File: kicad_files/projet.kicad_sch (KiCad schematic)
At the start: 32 parts, among them J1 STLink V3, J4 USB_B_Micro, J5 Conn_01x04, J6 Conn_01x02, Q1 BC817, Q2 BC807, Q3 NMOS, Q4 PMOS, SW1 SW_Omron_B3FS, SW2 Reset, U1 STM32G031K8Tx, U2 MCP4901, U3 LM1117MP-3.3, U4 TLV2372, U5 CD4066BM, U6 MCP4131-xxxx-P, U7 MCP4901

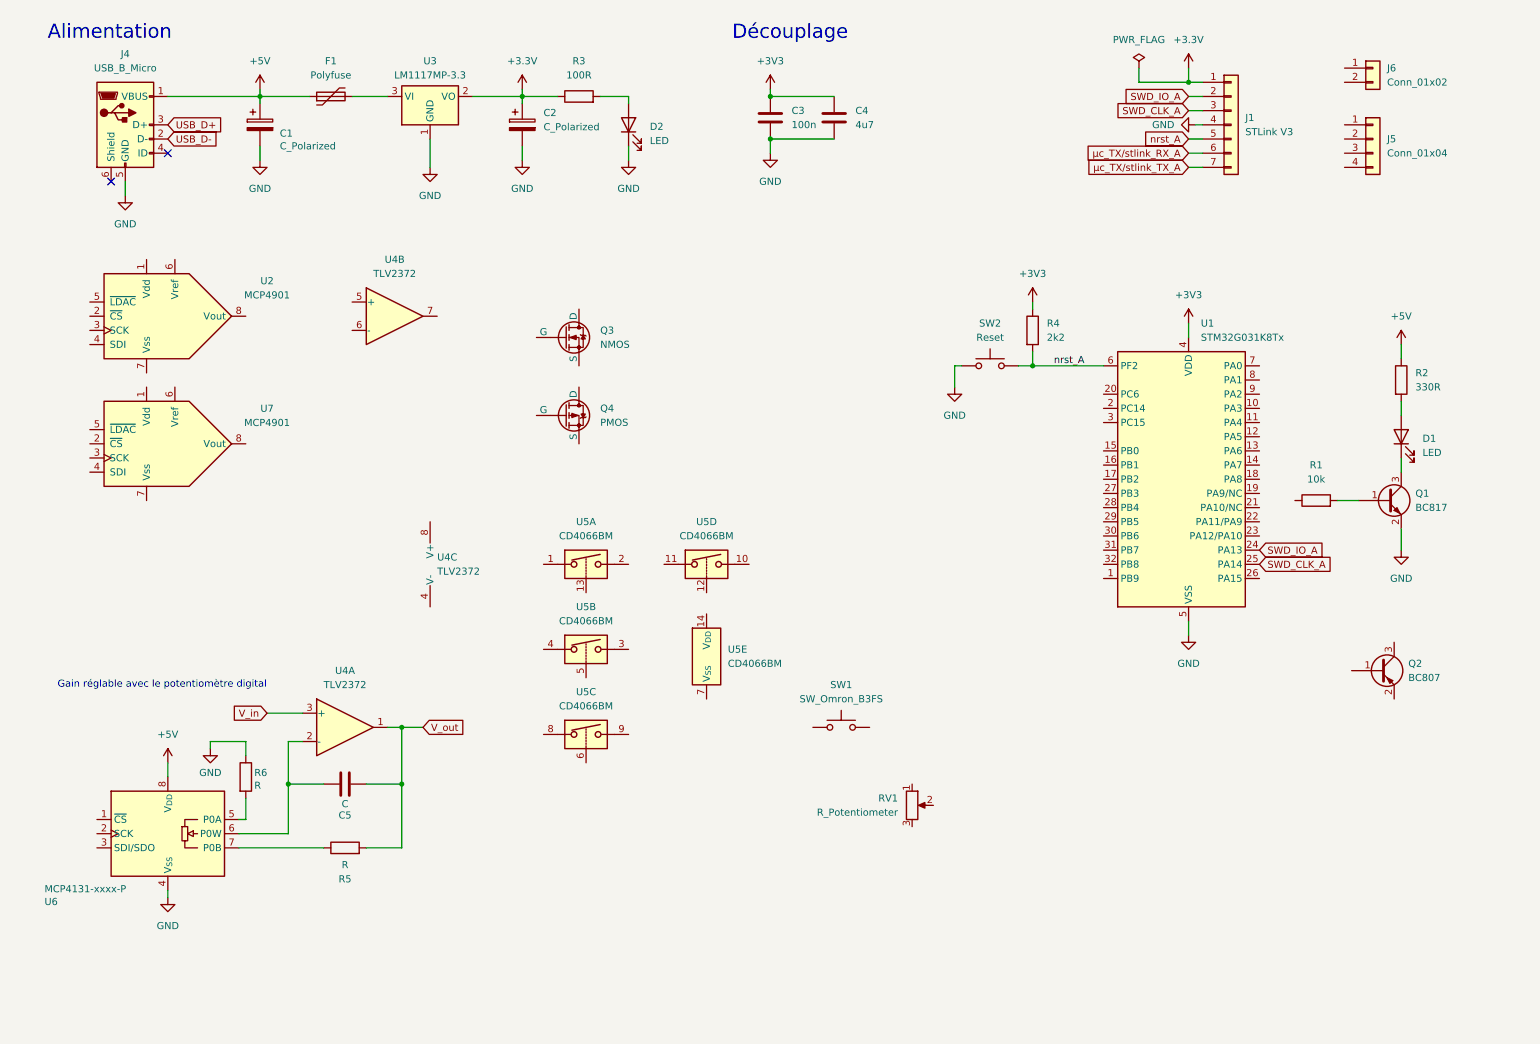
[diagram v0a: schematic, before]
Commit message: circuit
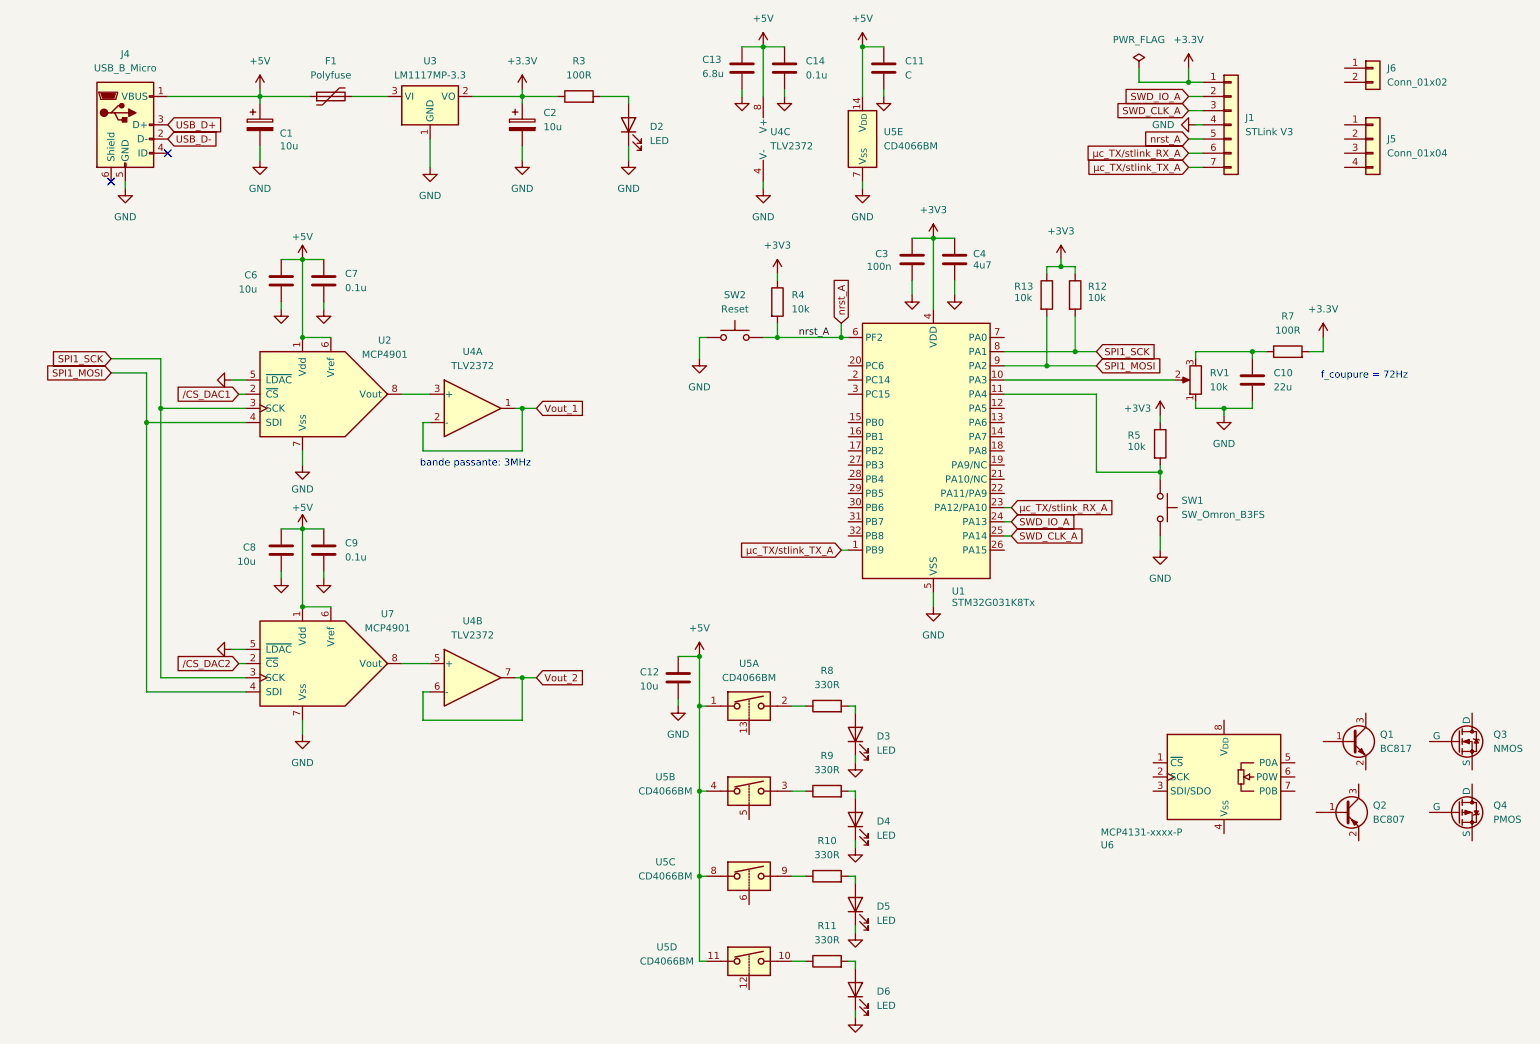
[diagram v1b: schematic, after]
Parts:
- removed C5: C, symbol Device:C
- removed D1: LED, symbol Device:LED
- removed R1: 10k, symbol Device:R
- removed R2: 330R, symbol Device:R
- removed R6: R, symbol Device:R
- added C10: 22u, symbol Device:C
- added C11: C, symbol Device:C
- added C12, C6, C8: 10u, symbol Device:C
- added C13: 6.8u, symbol Device:C
- added C14, C7, C9: 0.1u, symbol Device:C
- added D3, D4, D5, D6: LED, symbol Device:LED
- added R10, R11, R8, R9: 330R, symbol Device:R
- added R12, R13: 10k, symbol Device:R
- added R7: 100R, symbol Device:R
- C1, C2: value C_Polarized -> 10u
- R4: value 2k2 -> 10k
- R5: value R -> 10k
- RV1: value R_Potentiometer -> 10k
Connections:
- net V_in is gone; now on an unnamed net: U4.3 (+)
- net +3.3V: now also R7.2
- net +3V3: now also R5.1, R12.1, R13.1
- net +5V: now also U2.1 (Vdd), U2.6 (Vref), U4.8 (V+), U5.1, U5.11, U5.14 (V_{DD}), U5.4, U5.8, U7.1 (Vdd), U7.6 (Vref), C11.1, C12.1, C13.1, C14.1, C6.1, C7.1, C8.1, C9.1; no longer U6.8 (V_{DD})
- net GND: now also RV1.1, SW1.2, U2.7 (Vss), U4.4 (V-), U5.7 (V_{SS}), U7.7 (Vss), C10.2, C12.2; no longer C3.2, C4.2, Q1.2 (E), U6.4 (V_{SS})
- net µc_TX/stlink_RX_A: now also U1.23 (PA12/PA10)
- net µc_TX/stlink_TX_A: now also U1.1 (PB9)
- net at SW1.1: now also R5.2, U1.11 (PA4)
- net at U6.7 (P0B): no longer R5.1
- net at U1.10 (PA3): now also RV1.2
- net SPI1_SCK: now reaches U1.8 (PA1)
- net SPI1_SCK: now also U2.3 (SCK), U7.3 (SCK), R12.2
- net SPI1_MOSI: now reaches U1.9 (PA2)
- net SPI1_MOSI: now also U2.4 (SDI), U7.4 (SDI), R13.2
- net at U6.6 (P0W): no longer U4.2 (-)
- net at RV1.3: now also C10.1, R7.1
- net at U4.5 (+): now also U7.8 (Vout)
- net Vout_2: now reaches U4.6 (-)
- net Vout_2: now also U4.7
- net /CS_DAC1: now reaches U2.2 (~{CS})
- net at U5.3: now also R9.1
- net at U5.2: now also R8.1
- net at U5.10: now also R11.1
- net at U5.9: now also R10.1
- net /CS_DAC2: now reaches U7.2 (~{CS})
- net V_out renamed Vout_1
- net Vout_1: now also U4.2 (-); no longer R5.2
- new net: D3.2 (A), R8.2
- new net: D4.2 (A), R9.2
- new net: D6.2 (A), R11.2
- new net: D5.2 (A), R10.2
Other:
- note added: "bande passante: 3MHz"
- note added: "f_coupure = 72Hz"
- note removed: "Alimentation"
- note removed: "Découplage"
- note removed: "Gain réglable avec le potentiomètre digital"
- moved on the sheet: C3, C4, Q1, Q2, Q3, Q4, R4, RV1, SW1, SW2, U1, U2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

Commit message: circuit
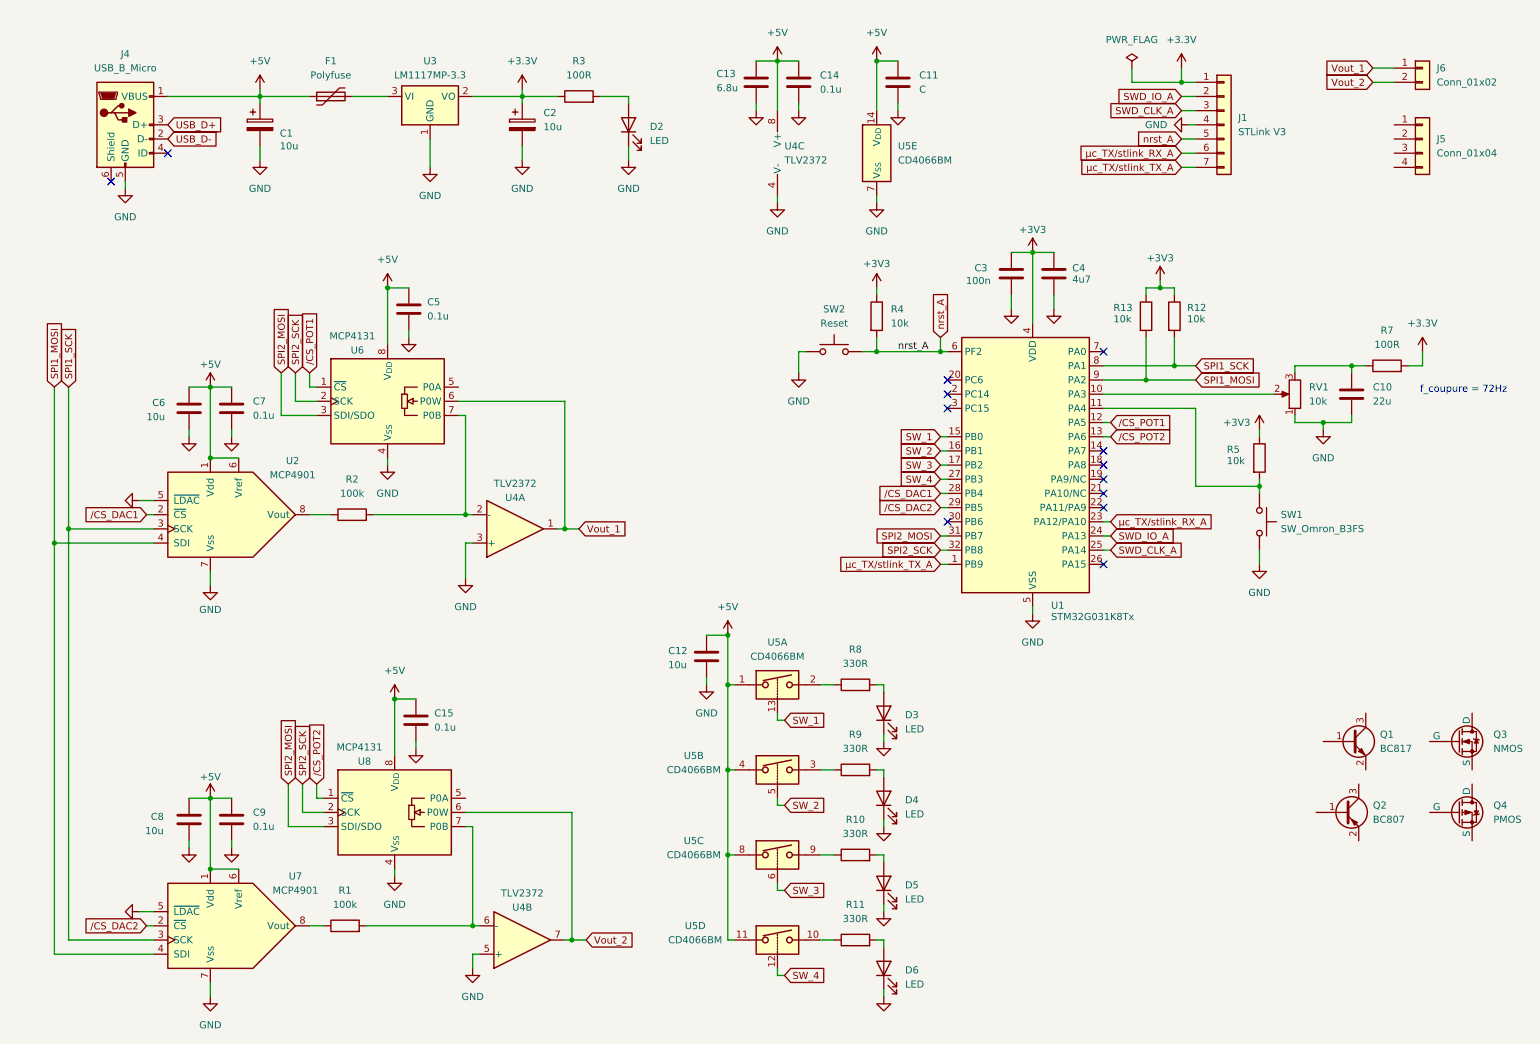
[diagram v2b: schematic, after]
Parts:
- added C15, C5: 0.1u, symbol Device:C
- added R1, R2: 100k, symbol Device:R
- added U8: MCP4131, Package_DIP:DIP-8_W7.62mm, symbol Potentiometer_Digital:MCP4131-xxxx-P
- U6: value MCP4131-xxxx-P -> MCP4131
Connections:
- net +5V: now also U6.8 (V_{DD}), C15.1, C5.1, U8.8 (V_{DD})
- net GND: now also U4.3 (+), U4.5 (+), U6.4 (V_{SS}), U8.4 (V_{SS})
- net Vout_1: now also J6.1 (Pin_1), U6.6 (P0W); no longer U4.2 (-)
- net Vout_2: now also J6.2 (Pin_2), U8.6 (P0W); no longer U4.6 (-)
- net /CS_DAC1: now also U1.28 (PB4)
- net /CS_DAC2: now also U1.29 (PB5)
- net /CS_POT1: now reaches U1.12 (PA5)
- net /CS_POT1: now also U6.1 (~{CS})
- net /CS_POT2: now reaches U1.13 (PA6)
- net /CS_POT2: now also U8.1 (~{CS})
- net SW_1: now reaches U1.15 (PB0)
- net SW_1: now also U5.13
- net SW_2: now reaches U1.16 (PB1)
- net SW_2: now also U5.5
- net SW_3: now reaches U1.17 (PB2)
- net SW_3: now also U5.6
- net SW_4: now reaches U1.27 (PB3)
- net SW_4: now also U5.12
- net SPI2_MOSI: now reaches U1.31 (PB7)
- net SPI2_MOSI: now also U6.3 (SDI/SDO), U8.3 (SDI/SDO)
- net SPI2_SCK: now reaches U1.32 (PB8)
- net SPI2_SCK: now also U6.2 (SCK), U8.2 (SCK)
- net at U2.8 (Vout): now also R2.1; no longer U4.3 (+)
- net at U7.8 (Vout): now also R1.1; no longer U4.5 (+)
- net at U6.7 (P0B): now also U4.2 (-), R2.2
- new net: R1.2, U4.6 (-), U8.7 (P0B)
- no-connect marks 2 -> 13
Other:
- note removed: "bande passante: 3MHz"
- moved on the sheet: C10, C11, C12, C13, C14, C3, C4, C6, C7, C8, C9, D3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

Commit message: schema et datasheets
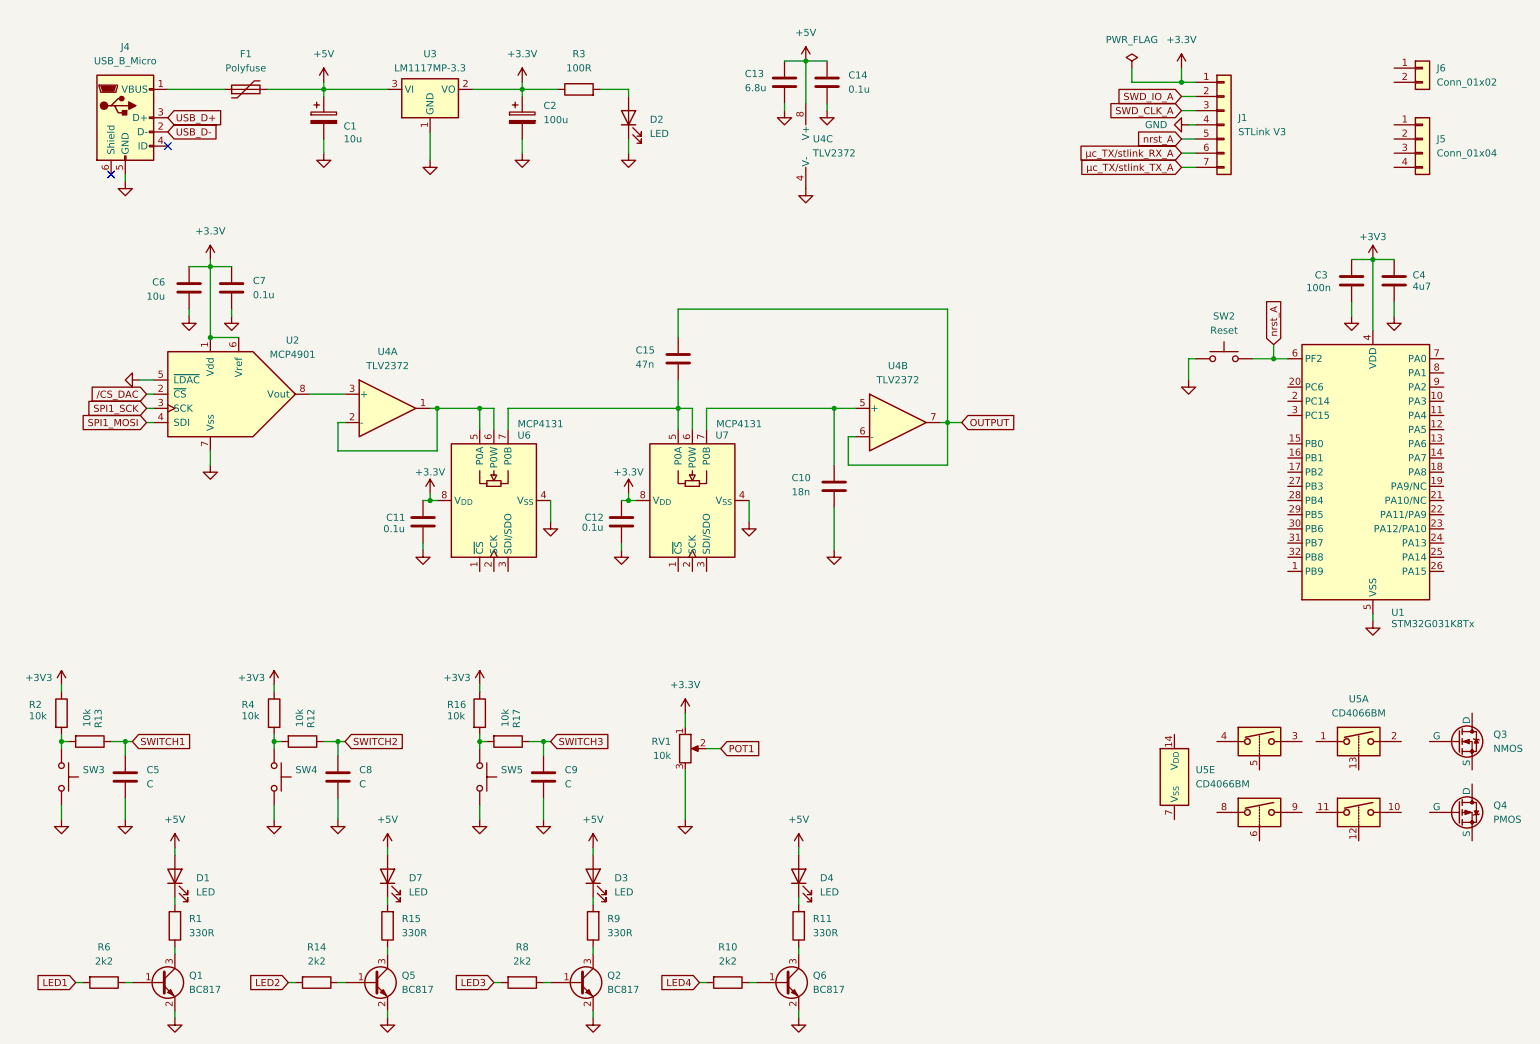
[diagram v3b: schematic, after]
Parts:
- removed D5, D6: LED, symbol Device:LED
- removed Q2: BC807, Package_TO_SOT_SMD:SOT-23, symbol Transistor_BJT:BC807
- removed R5: 10k, symbol Device:R
- removed R7: 100R, symbol Device:R
- removed SW1: SW_Omron_B3FS, symbol Switch:SW_Omron_B3FS
- removed U7: MCP4901, symbol Analog_DAC:MCP4901
- removed U8: MCP4131, Package_DIP:DIP-8_W7.62mm, symbol Potentiometer_Digital:MCP4131-xxxx-P
- added D1, D7: LED, symbol Device:LED
- added Q2, Q5, Q6: BC817, Package_TO_SOT_SMD:SOT-23, symbol Transistor_BJT:BC817
- added R14, R6: 2k2, symbol Device:R
- added R15: 330R, symbol Device:R
- added R16, R17: 10k, symbol Device:R
- added SW3, SW4, SW5: SW_Omron_B3FS, symbol Switch:SW_Omron_B3FS
- added U7: MCP4131, Package_DIP:DIP-8_W7.62mm, symbol Potentiometer_Digital:MCP4131-xxxx-P
- C10: value 22u -> 18n
- C11: value C -> 0.1u
- C12: value 10u -> 0.1u
- C15: value 0.1u -> 47n
- C2: value 10u -> 100u
- C5, C9: value 0.1u -> C
- C8: value 10u -> C
- R1: value 100k -> 330R
- R10, R8: value 330R -> 2k2
- R2: value 100k -> 10k
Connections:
- net +3.3V: now also C11.2, C12.1, C6.1, C7.1, RV1.1, U2.1 (Vdd), U2.6 (Vref), U6.8 (V_{DD}), U7.8 (V_{DD})
- net +3V3: now also R2.1, R16.1; no longer R12.1, R13.1
- net +5V: now also D3.2 (A), D4.2 (A), F1.2, U3.3 (VI), D1.2 (A), D7.2 (A); no longer C11.1, C12.1, C15.1, C5.1, C6.1, C7.1, C8.1, C9.1, F1.1, J4.1 (VBUS), U2.1 (Vdd), U2.6 (Vref), U5.1, U5.11, U5.14 (V_{DD}), U5.4, U5.8, U6.8 (V_{DD})
- net GND: no longer C1.2, C10.2, C12.2, C2.2, D2.1 (K), J4.5 (GND), RV1.1, SW2.1, U1.5 (VSS), U2.7 (Vss), U3.1 (GND), U4.3 (+), U4.4 (V-), U4.5 (+), U5.7 (V_{SS}), U6.4 (V_{SS})
- net SPI1_MOSI: no longer R13.2, U1.9 (PA2)
- net SPI1_SCK: no longer R12.2, U1.8 (PA1)
- net SWD_CLK_A: no longer U1.25 (PA14)
- net SWD_IO_A: no longer U1.24 (PA13)
- net nrst_A: no longer R4.2
- net µc_TX/stlink_RX_A: no longer U1.23 (PA12/PA10)
- net µc_TX/stlink_TX_A: no longer U1.1 (PB9)
- net at R1.2: now also D1.1 (K); no longer U4.6 (-)
- net OUTPUT: now reaches C15.2
- net OUTPUT: now also U4.6 (-), U4.7
- net at U1.10 (PA3): no longer RV1.2
- net at U5.2: no longer R8.1
- net LED3: now reaches R8.2
- net LED3: no longer D3.2 (A)
- net at C10.1: no longer RV1.3
- net at D3.1 (K): now also R9.2
- net at U6.5 (P0A): now also U4.1, U4.2 (-), U6.6 (P0W)
- net at D4.1 (K): now also R11.2
- net at U2.8 (Vout): now also U4.3 (+); no longer R2.1
- net at R11.1: now also Q6.3 (C); no longer U5.10
- net at R9.1: now also Q2.3 (C); no longer U5.3
- net at Q1.1 (B): now also R6.1
- net at Q1.3 (C): now also R1.1
- net at R10.1: now also Q6.1 (B); no longer U5.9
- net LED4: now reaches R10.2
- net SPI2_MOSI: no longer names the net of U6.3 (SDI/SDO)
- net SPI2_MOSI: no longer U1.31 (PB7)
- net SPI2_SCK: no longer names the net of U6.2 (SCK)
- net SPI2_SCK: no longer U1.32 (PB8)
- net SW_1: no longer names the net of U1.15 (PB0)
- net SW_1: no longer U5.13
- net SW_2: no longer names the net of U1.16 (PB1)
- net SW_2: no longer U5.5
- net SW_3: no longer names the net of U1.17 (PB2)
- net SW_3: no longer U5.6
- net SW_4: no longer names the net of U1.27 (PB3)
- net SW_4: no longer U5.12
- removed net Vout_1: J6.1 (Pin_1), U4.1, U6.6 (P0W)
- net Vout_2: no longer names the net of J6.2 (Pin_2)
- net Vout_2: no longer U4.7
- net /CS_DAC1: no longer names the net of U1.28 (PB4)
- net /CS_DAC1: no longer U2.2 (~{CS})
- net /CS_DAC2: no longer names the net of U1.29 (PB5)
- net /CS_POT1: no longer names the net of U6.1 (~{CS})
- net /CS_POT1: no longer U1.12 (PA5)
- net /CS_POT2: no longer names the net of U1.13 (PA6)
- new net: R13.2, R2.2, SW3.1
- new net: R16.2, R17.2, SW5.1
- new net: C15.1, U6.7 (P0B), U7.5 (P0A), U7.6 (P0W)
- new net: C10.2, U4.5 (+), U7.7 (P0B)
- new net: R12.2, R4.2, SW4.1
- new net: Q5.3 (C), R15.1
- new net: D7.1 (K), R15.2
- new net: Q5.1 (B), R14.1
- new net: Q2.1 (B), R8.1
- new net: F1.1, J4.1 (VBUS)
- new net LED1: R6.2
- new net LED2: R14.2
- new net POT1: RV1.2
- new net SWITCH1: C5.1, R13.1
- new net SWITCH2: C8.1, R12.1
- new net SWITCH3: C9.1, R17.1
- new net /CS_DAC: U2.2 (~{CS})
- no-connect marks 13 -> 2
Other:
- note removed: "f_coupure = 72Hz"
- moved on the sheet: C1, C13, C14, C2, C3, C4, C6, C7, D2, J4, Q1, R3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
